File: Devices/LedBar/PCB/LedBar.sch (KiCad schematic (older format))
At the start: 6 parts

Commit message: Renamed libraries
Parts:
- MB101, MB102, MB103, MB104, MB106: footprint AmbientLight:MouseBit -> RGBW-Bar:MouseBit; symbol AmbientLight:MouseBit -> RGBW-Bar:MouseBit
- MB105: footprint AmbientLight:MouseBit_modified1 -> RGBW-Bar:MouseBit_modified1; symbol AmbientLight:MouseBit -> RGBW-Bar:MouseBit
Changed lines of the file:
@@
 	3500 1500 3500 4750
 $Comp
-L AmbientLight:MouseBit MB101
+L RGBW-Bar:MouseBit MB101
 U 1 1 618FDB69
 P 1450 1000
 F 0 "MB101" H 1728 1046 50  0000 L CNN
 F 1 "MouseBit" H 1728 955 50  0000 L CNN
-F 2 "AmbientLight:MouseBit" H 1370 1420 50  0001 C CNN
+F 2 "RGBW-Bar:MouseBit" H 1370 1420 50  0001 C CNN
 F 3 "" H 1450 940 50  0001 C CNN
 	1    1450 1000
@@
 $EndComp
 $Comp
-L AmbientLight:MouseBit MB102
+L RGBW-Bar:MouseBit MB102
 U 1 1 61901AE5
 P 1450 1300
 F 0 "MB102" H 1728 1346 50  0000 L CNN
 F 1 "MouseBit" H 1728 1255 50  0000 L CNN
-F 2 "AmbientLight:MouseBit" H 1370 1720 50  0001 C CNN
+F 2 "RGBW-Bar:MouseBit" H 1370 1720 50  0001 C CNN
 F 3 "" H 1450 1240 50  0001 C CNN
 	1    1450 1300
@@
 $EndComp
 $Comp
-L AmbientLight:MouseBit MB103
+L RGBW-Bar:MouseBit MB103
 U 1 1 619021A7
 P 1450 1600
 F 0 "MB103" H 1728 1646 50  0000 L CNN
 F 1 "MouseBit" H 1728 1555 50  0000 L CNN
-F 2 "AmbientLight:MouseBit" H 1370 2020 50  0001 C CNN
+F 2 "RGBW-Bar:MouseBit" H 1370 2020 50  0001 C CNN
 F 3 "" H 1450 1540 50  0001 C CNN
 	1    1450 1600
@@
 $EndComp
 $Comp
-L AmbientLight:MouseBit MB104
+L RGBW-Bar:MouseBit MB104
 U 1 1 61907DC7
 P 1450 1900
 F 0 "MB104" H 1728 1946 50  0000 L CNN
 F 1 "MouseBit" H 1728 1855 50  0000 L CNN
-F 2 "AmbientLight:MouseBit" H 1370 2320 50  0001 C CNN
+F 2 "RGBW-Bar:MouseBit" H 1370 2320 50  0001 C CNN
 F 3 "" H 1450 1840 50  0001 C CNN
 	1    1450 1900
@@
 $EndComp
 $Comp
-L AmbientLight:MouseBit MB105
+L RGBW-Bar:MouseBit MB105
 U 1 1 619FF750
 P 1450 2200
 F 0 "MB105" H 1728 2246 50  0000 L CNN
 F 1 "MouseBit" H 1728 2155 50  0000 L CNN
-F 2 "AmbientLight:MouseBit_modified1" H 1370 2620 50  0001 C CNN
+F 2 "RGBW-Bar:MouseBit_modified1" H 1370 2620 50  0001 C CNN
 F 3 "" H 1450 2140 50  0001 C CNN
 	1    1450 2200
@@
 $EndComp
 $Comp
-L AmbientLight:MouseBit MB106
+L RGBW-Bar:MouseBit MB106
 U 1 1 619FFB38
 P 1450 2500
 F 0 "MB106" H 1728 2546 50  0000 L CNN
 F 1 "MouseBit" H 1728 2455 50  0000 L CNN
-F 2 "AmbientLight:MouseBit" H 1370 2920 50  0001 C CNN
+F 2 "RGBW-Bar:MouseBit" H 1370 2920 50  0001 C CNN
 F 3 "" H 1450 2440 50  0001 C CNN
 	1    1450 2500

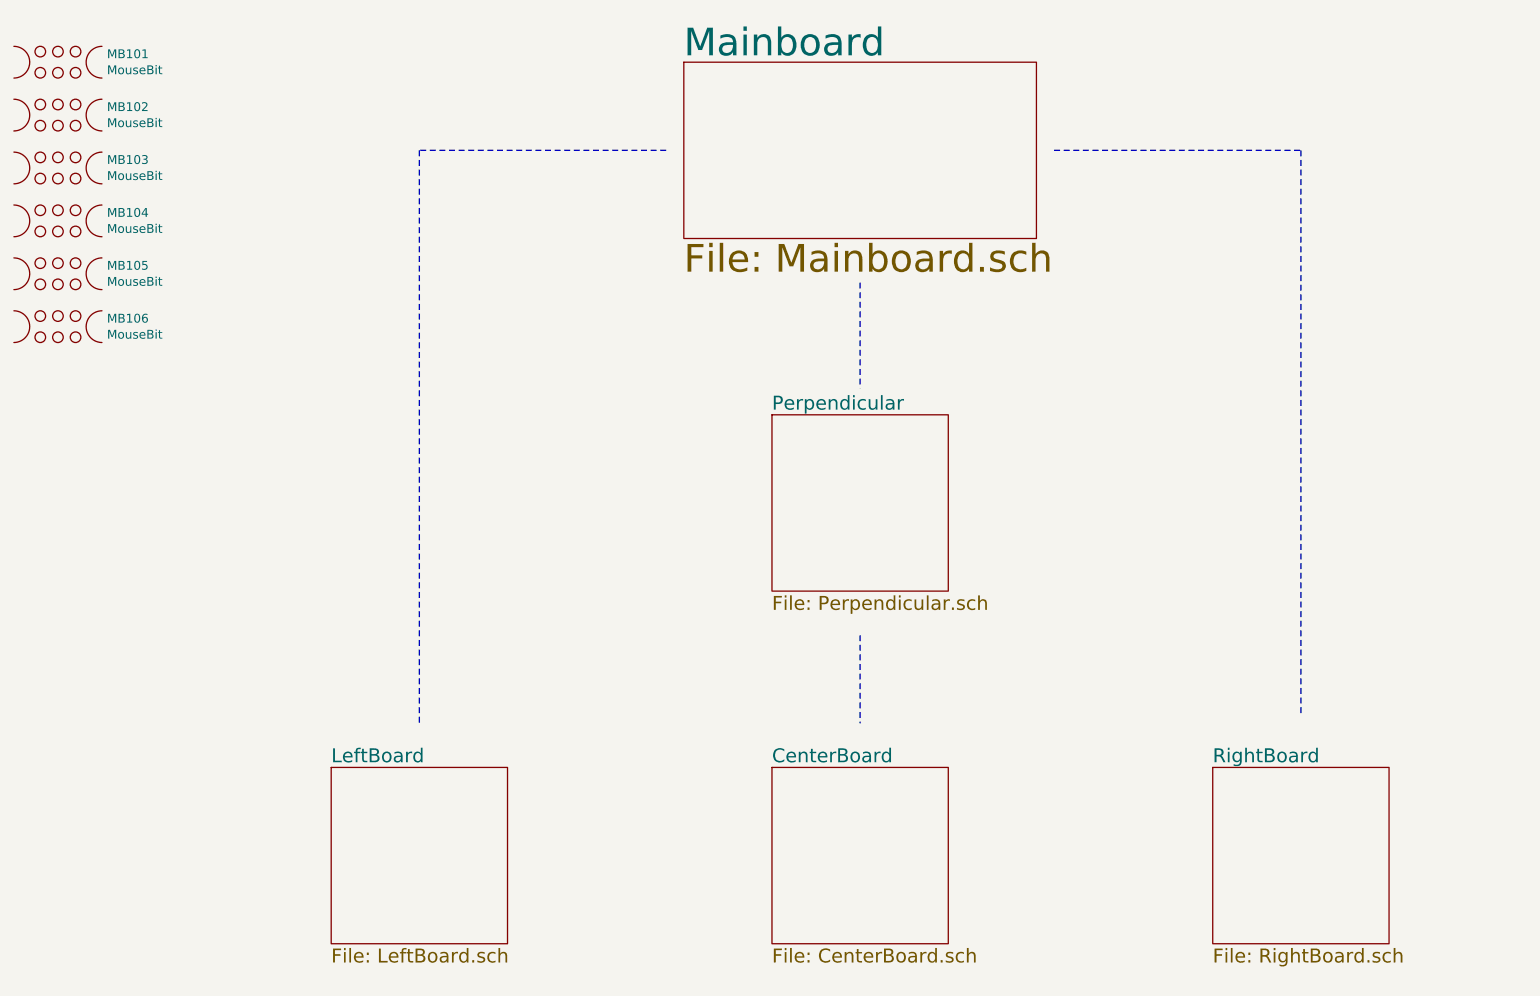
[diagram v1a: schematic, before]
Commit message: Cosmetic changes to shematics
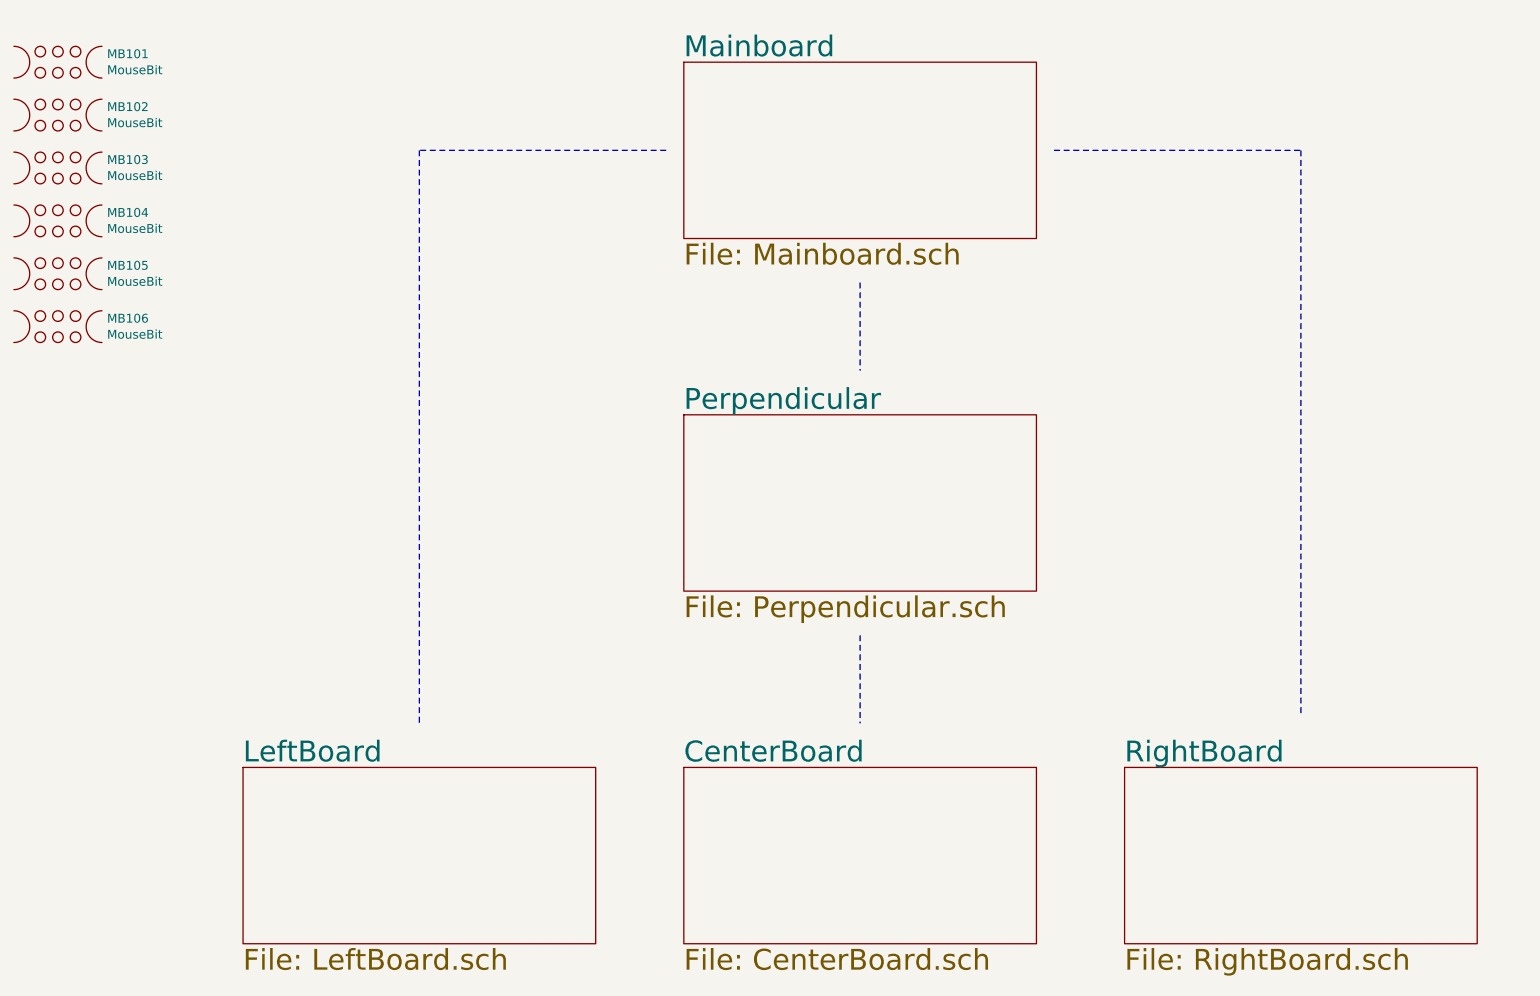
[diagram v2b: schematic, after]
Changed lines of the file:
@@
 Rev "0.1"
 Comp "Roel Drost"
-Comment1 ""
+Comment1 "GNU General Public License v3.0"
 Comment2 ""
 Comment3 ""
-Comment4 ""
+Comment4 "4 channel RGBW LED bar, Arduino compatible with isolated half duplex RS485."
 $EndDescr
-Wire Notes Line
-	6000 2250 6000 2850
 $Sheet
 S 5000 1000 2000 1000
 U 617A8CB5
-F0 "Mainboard" 157
-F1 "Mainboard.sch" 157
+F0 "Mainboard" 118
+F1 "Mainboard.sch" 118
 $EndSheet
 Wire Notes Line
@@
 	6000 4250 6000 4750
 $Sheet
-S 5500 3000 1000 1000
-U 6187FE9B
-F0 "Perpendicular" 79
-F1 "Perpendicular.sch" 79
+S 2500 5000 2000 1000
+U 618804D0
+F0 "LeftBoard" 118
+F1 "LeftBoard.sch" 118
 $EndSheet
 $Sheet
-S 3000 5000 1000 1000
-U 618804D0
-F0 "LeftBoard" 79
-F1 "LeftBoard.sch" 79
+S 5000 5000 2000 1000
+U 6188050F
+F0 "CenterBoard" 118
+F1 "CenterBoard.sch" 118
 $EndSheet
 $Sheet
-S 5500 5000 1000 1000
-U 6188050F
-F0 "CenterBoard" 79
-F1 "CenterBoard.sch" 79
-$EndSheet
-$Sheet
-S 8000 5000 1000 1000
+S 7500 5000 2000 1000
 U 6188055C
-F0 "RightBoard" 79
-F1 "RightBoard.sch" 79
+F0 "RightBoard" 118
+F1 "RightBoard.sch" 118
 $EndSheet
 Wire Notes Line
@@
 	1    0    0    -1
 $EndComp
+$Sheet
+S 5000 3000 2000 1000
+U 6187FE9B
+F0 "Perpendicular" 118
+F1 "Perpendicular.sch" 118
+$EndSheet
+Wire Notes Line
+	6000 2250 6000 2750
 $EndSCHEMATC
